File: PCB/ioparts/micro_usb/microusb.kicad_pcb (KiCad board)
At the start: 2 copper layers, 13.5 x 8 mm, 2 parts, among them J1 USB_B_Micro, J3 Conn_01x04

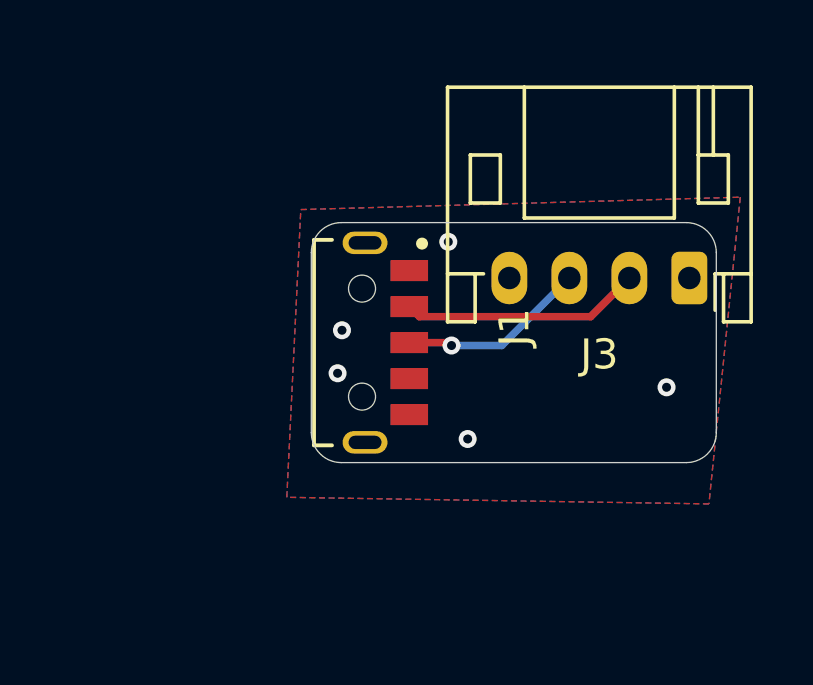
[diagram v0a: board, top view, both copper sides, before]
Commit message: misc pcbs
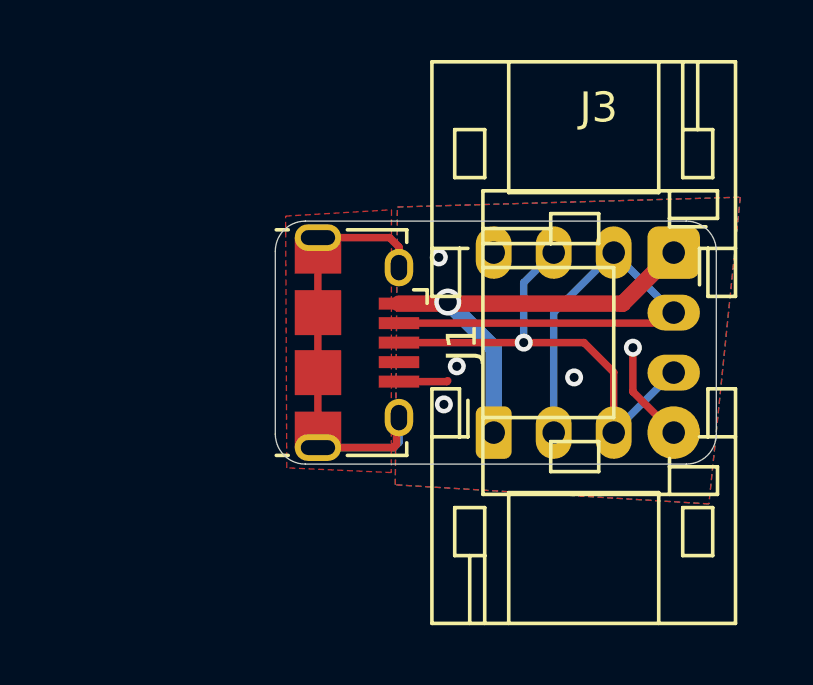
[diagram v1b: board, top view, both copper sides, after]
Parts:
- J1: footprint ioparts:HRO_U-G-M5WS-W-01 -> Connector_USB:USB_Micro-B_Amphenol_10118194_Horizontal
- moved J3 0.99 mm to (118.1, 47.0)
- moved J1 0.17 mm to (107.5, 50.0)
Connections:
- net VBUS_MICRO renamed VBUS
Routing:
- net SHIELD: track 0.00 -> 17.6 mm
- net VBUS: track 0.00 -> 14.8 mm, vias 0 -> 1
- net DM_MICRO: track 8.01 -> 18.5 mm
- net DP_MICRO: track 6.31 -> 15.8 mm
- net GND1: track 0.00 -> 5.03 mm
- added copper zone on F.Cu, net SHIELD
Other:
- board size 13.5 x 8 mm -> 14.7 x 8.1 mm

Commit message: misc pcbs
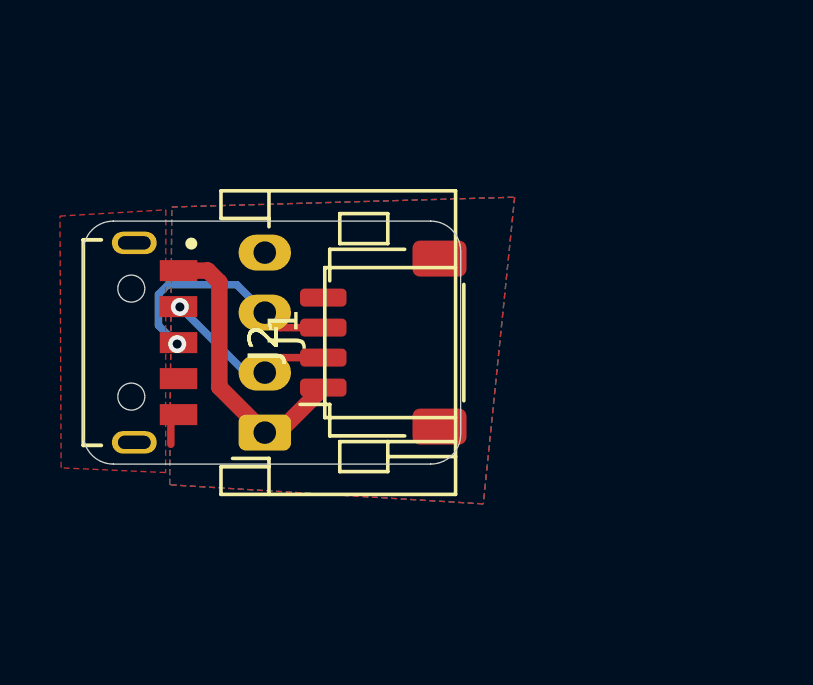
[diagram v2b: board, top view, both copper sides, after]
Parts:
- added J2: Conn_01x04, Connector_JST:JST_SH_SM04B-SRSS-TB_1x04-1MP_P1.00mm_Horizontal, F.Cu at (108.4, 50.0)
- J1: footprint Connector_USB:USB_Micro-B_Amphenol_10118194_Horizontal -> ioparts:HRO_U-G-M5WS-W-01
- moved J3 14.9 mm to (104.4, 53.0), turned to 90 degrees
- moved J1 7.52 mm to (100.0, 50.0)
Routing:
- net SHIELD: track 17.6 -> 0.00 mm
- net DM_MICRO: track 18.5 -> 5.25 mm, vias 0 -> 1
- net DP_MICRO: track 15.8 -> 8.13 mm
- net VBUS: track 14.8 -> 9.01 mm, vias 1 -> 0
- net GND1: track 5.03 -> 0.81 mm, vias 5 -> 0
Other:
- board size 14.7 x 8.1 mm -> 12.6 x 8.1 mm
